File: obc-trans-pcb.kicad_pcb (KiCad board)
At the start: 4 copper layers, 95.9 x 90.2 mm, 31 parts, among them IC1 DS3234, J1 H1, J2 H2, J3 H_EPS, J4 DEBUGGING PORT, J5 PROGRAMMING PORT, SW1 SW_RST, U1 SN65HVD230, U2 ATMEGA32M1-MU, U3 SST25VF016B, U4 SST25VF016B, U5 SST25VF016B, Y1 8 MHz

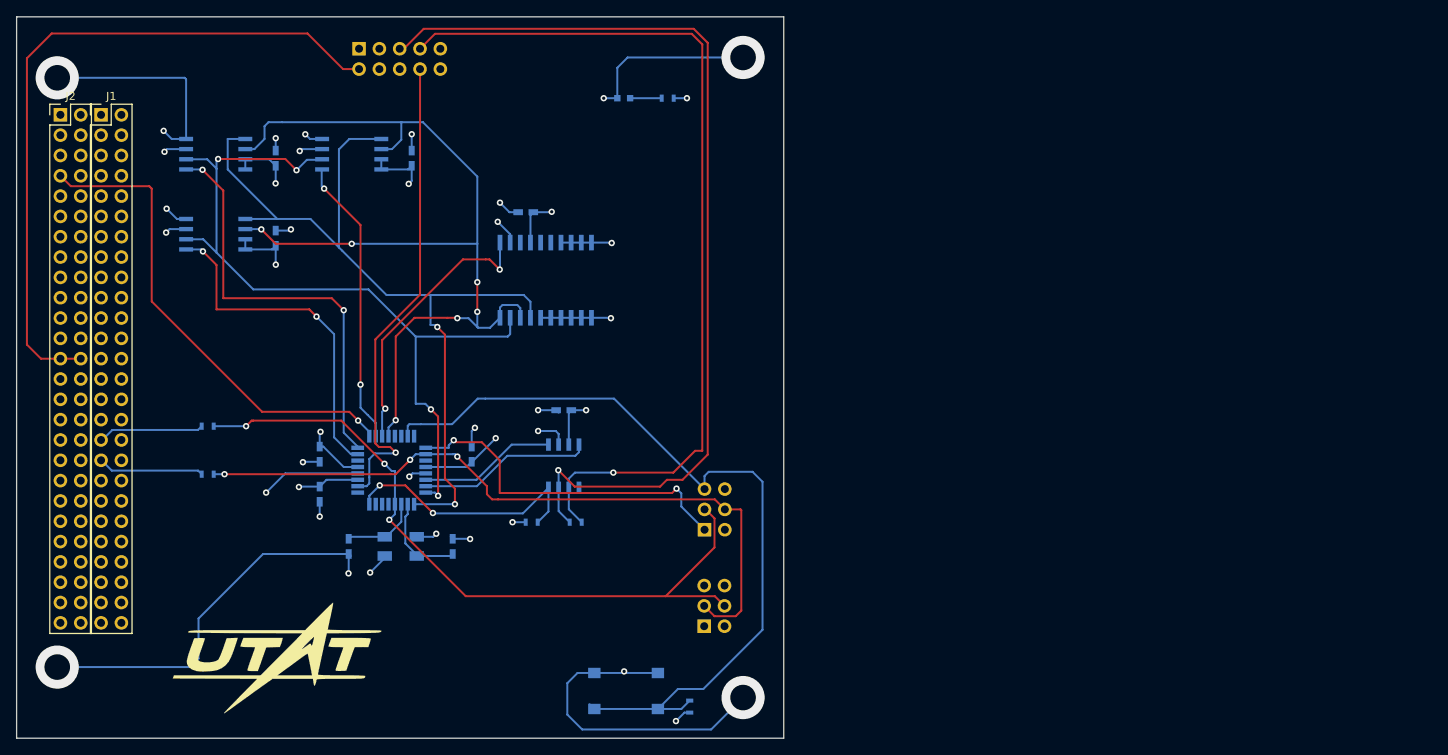
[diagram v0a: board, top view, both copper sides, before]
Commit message: Revert "vias smaller"
This reverts commit cac4902e6433adb27f0d020128540fc5646aa025.
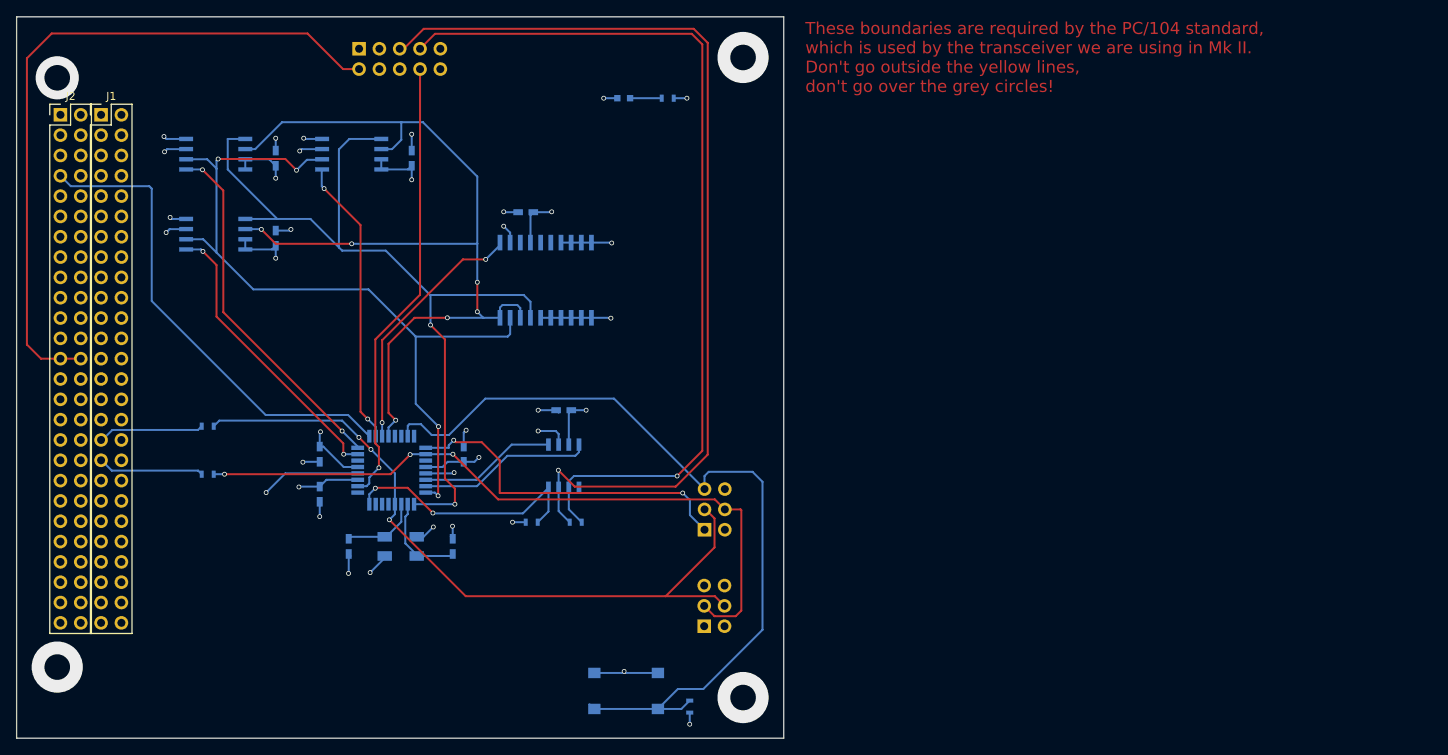
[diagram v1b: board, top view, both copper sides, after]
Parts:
- removed G***: LOGO, obc-trans-pcb:utat-logo
- moved C2 1.00 mm to (156.0, 104.5)
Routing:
- net GND: track 207.0 -> 83.2 mm
- net /CS_MEM2: track 52.8 -> 44.9 mm
- net /CS_MEM3: track 42.9 -> 36.6 mm
- net +3V3: track 73.4 -> 67.4 mm
- net /EPS_RST: track 60.4 -> 56.4 mm
- net /CS_RTC: track 35.4 -> 32.0 mm
- net /SCK: track 121.1 -> 119.0 mm
- net /RST: track 103.0 -> 104.1 mm
- net /MOSI_A: track 88.9 -> 87.9 mm
- net /MISO: track 101.4 -> 100.7 mm
- net /EN_UHF: track 60.7 -> 60.3 mm, vias 1 -> 0
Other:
- rule pad_to_mask_clearance: 0.25 -> 0.2
- board text added: "These boundaries are required by the PC/104 standard, which is used by the transceiver we are using in Mk II. Don't go outside the yellow lines, don't go over the grey circles!"

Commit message: vias smaller
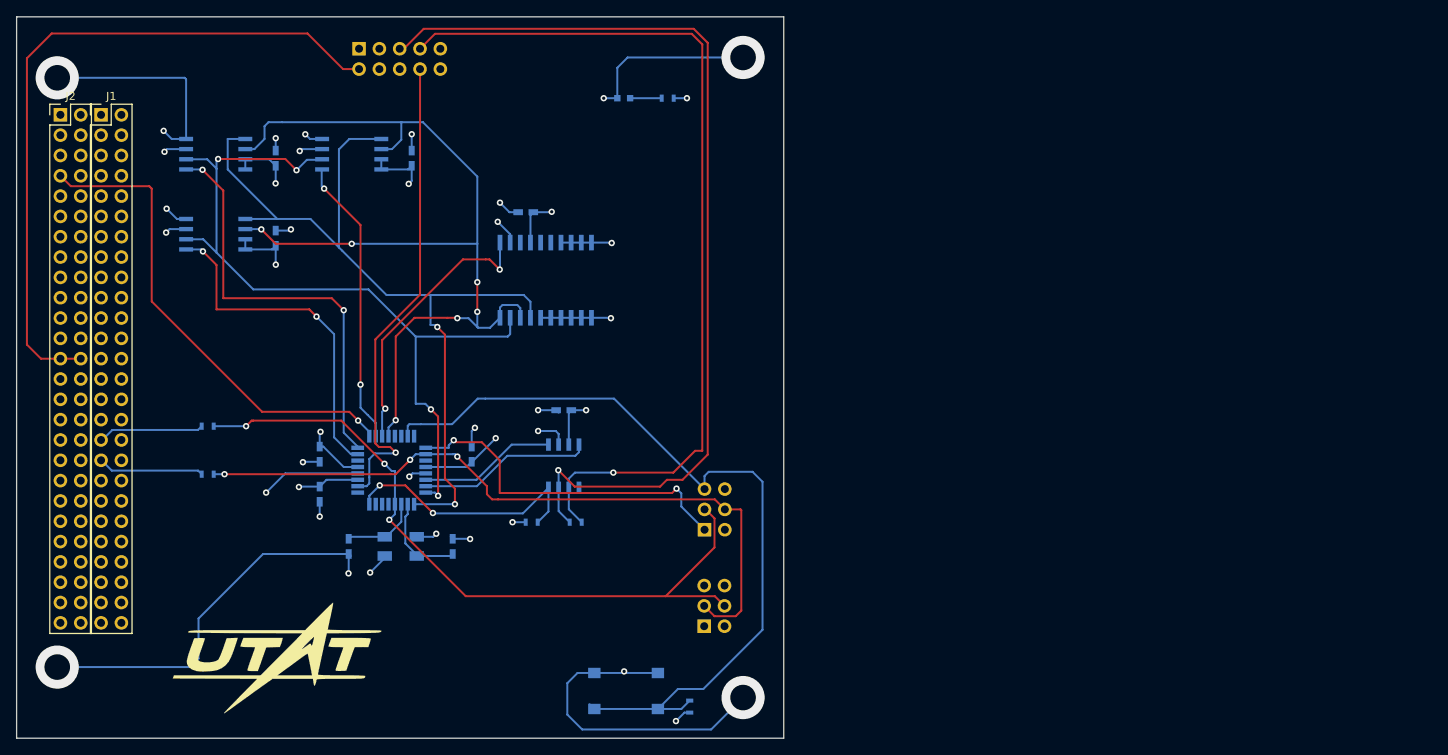
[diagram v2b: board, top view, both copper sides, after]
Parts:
- added G***: LOGO, obc-trans-pcb:utat-logo, F.Cu at (132.8, 129.6)
- moved C2 1.00 mm to (157.0, 104.5)
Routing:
- net GND: track 83.2 -> 207.0 mm
- net /CS_MEM2: track 44.9 -> 52.8 mm
- net /CS_MEM3: track 36.6 -> 42.9 mm
- net +3V3: track 67.4 -> 73.4 mm
- net /EPS_RST: track 56.4 -> 60.4 mm
- net /CS_RTC: track 32.0 -> 35.4 mm
- net /SCK: track 119.0 -> 121.1 mm
- net /RST: track 104.1 -> 103.0 mm
- net /MOSI_A: track 87.9 -> 88.9 mm
- net /MISO: track 100.7 -> 101.4 mm
- net /EN_UHF: track 60.3 -> 60.7 mm, vias 0 -> 1
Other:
- rule pad_to_mask_clearance: 0.2 -> 0.25
- board text removed: "These boundaries are required by the PC/104 standard, which is used by the transceiver we are using in Mk II. Don't go outside the yellow lines, don't go over the grey circles!"

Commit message: removed needless traces
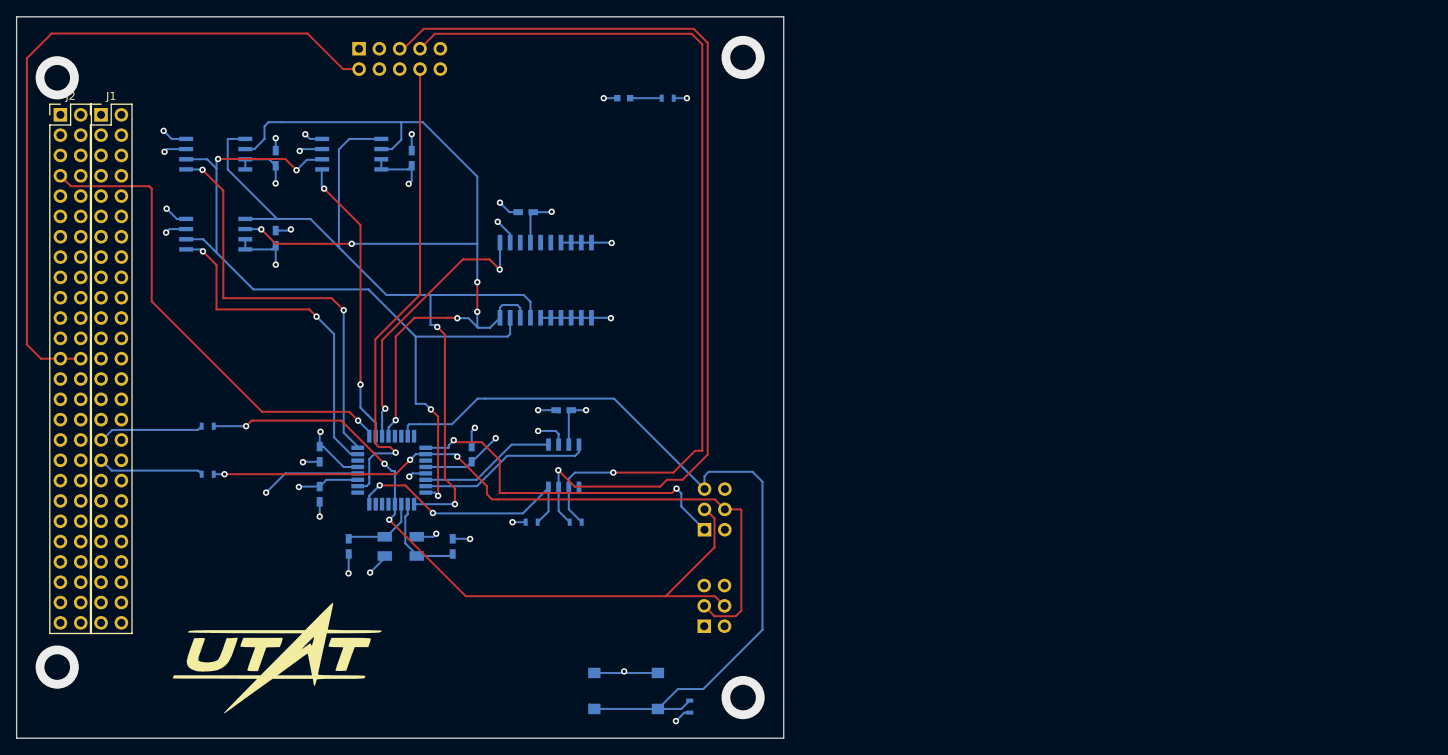
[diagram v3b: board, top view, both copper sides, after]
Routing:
- net GND: track 207.0 -> 87.3 mm
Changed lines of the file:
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@@
     (thickness 1.6)
     (drawings 4)
-    (tracks 494)
+    (tracks 478)
     (zones 0)
     (modules 31)
@@
   (gr_line (start 196 49.83) (end 100.11 49.83) (angle 90) (layer Edge.Cuts) (width 0.15))
   (gr_line (start 196 49.83) (end 196 140) (angle 90) (layer Edge.Cuts) (width 0.15))
-  (segment (start 141.625 116.975) (end 130.915 116.975) (width 0.25) (layer B.Cu) (net 1))
   (via (at 105.19 131.11) (size 5.4) (drill 3.2) (layers F.Cu B.Cu) (net 1))
-  (segment (start 121.78 131.11) (end 105.19 131.11) (width 0.25) (layer B.Cu) (net 1))
   (segment (start 122.85 130.04) (end 121.78 131.11) (width 0.25) (layer B.Cu) (net 1))
-  (segment (start 122.85 125.04) (end 122.85 130.04) (width 0.25) (layer B.Cu) (net 1))
-  (segment (start 130.915 116.975) (end 122.85 125.04) (width 0.25) (layer B.Cu) (net 1))
-  (segment (start 172.325 131.845554) (end 170.224446 131.845554) (width 0.25) (layer B.Cu) (net 1))
   (via (at 190.92 134.92) (size 5.4) (drill 3.2) (layers F.Cu B.Cu) (net 1))
-  (segment (start 186.93 138.91) (end 190.92 134.92) (width 0.25) (layer B.Cu) (net 1))
-  (segment (start 170.81 138.91) (end 186.93 138.91) (width 0.25) (layer B.Cu) (net 1))
-  (segment (start 168.95 137.05) (end 170.81 138.91) (width 0.25) (layer B.Cu) (net 1))
-  (segment (start 168.95 133.12) (end 168.95 137.05) (width 0.25) (layer B.Cu) (net 1))
-  (segment (start 170.224446 131.845554) (end 168.95 133.12) (width 0.25) (layer B.Cu) (net 1))
-  (segment (start 175.2 60) (end 175.2 56.2) (width 0.25) (layer B.Cu) (net 1))
   (via (at 190.92 54.91) (size 5.4) (drill 3.2) (layers F.Cu B.Cu) (net 1))
-  (segment (start 176.49 54.91) (end 190.92 54.91) (width 0.25) (layer B.Cu) (net 1))
-  (segment (start 175.2 56.2) (end 176.49 54.91) (width 0.25) (layer B.Cu) (net 1))
-  (segment (start 121.3 65.095) (end 121.3 57.64) (width 0.25) (layer B.Cu) (net 1))
   (via (at 105.19 57.45) (size 5.4) (drill 3.2) (layers F.Cu B.Cu) (net 1))
-  (segment (start 121.11 57.45) (end 105.19 57.45) (width 0.25) (layer B.Cu) (net 1))
-  (segment (start 121.3 57.64) (end 121.11 57.45) (width 0.25) (layer B.Cu) (net 1))
   (segment (start 161.805 78.05) (end 161.805 77.005) (width 0.25) (layer B.Cu) (net 1))
   (via (at 160.25 75.45) (size 0.8) (drill 0.4) (layers F.Cu B.Cu) (net 1))

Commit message: Revert "removed needless traces"
This reverts commit 13567706eda5130220792ebe949a07ef88a05d37.
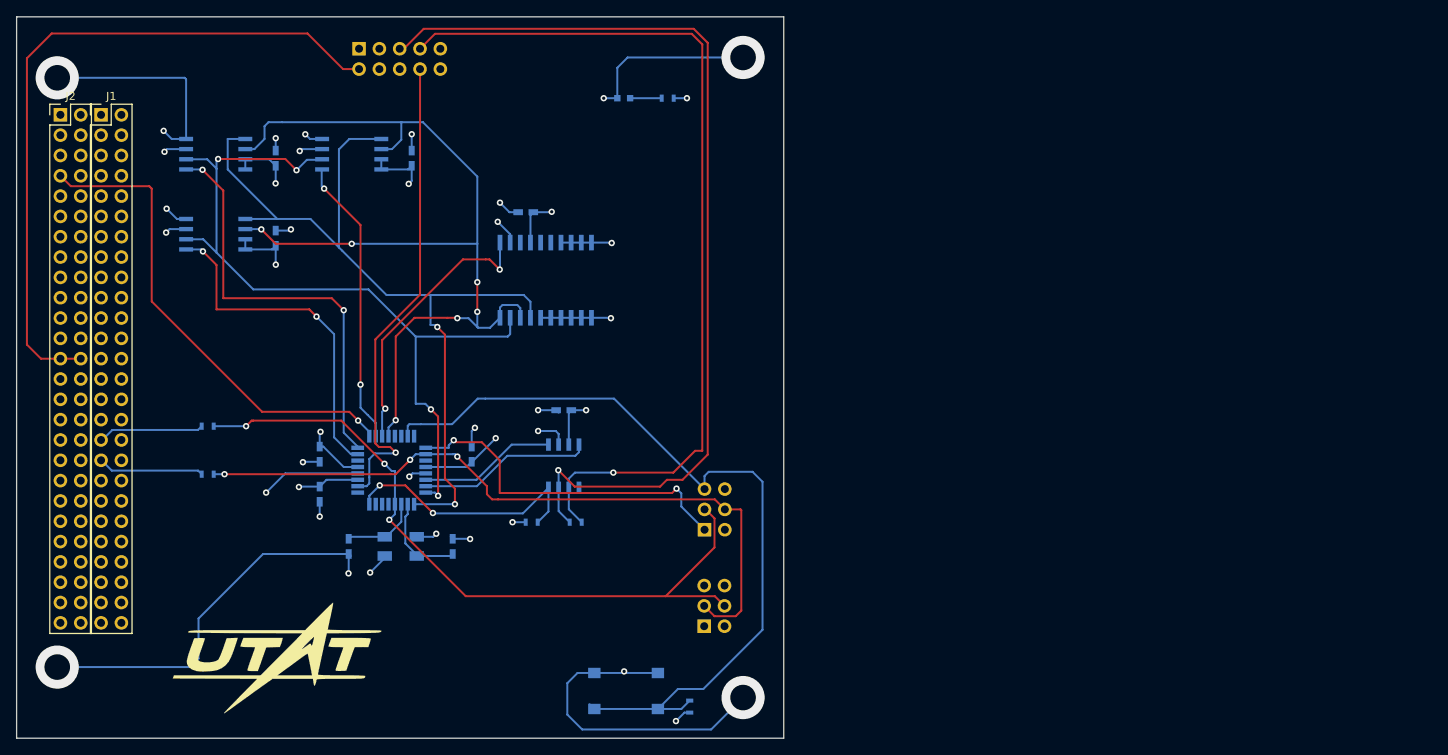
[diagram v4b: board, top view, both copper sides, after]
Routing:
- net GND: track 87.3 -> 207.0 mm
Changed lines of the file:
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@@
     (thickness 1.6)
     (drawings 4)
-    (tracks 478)
+    (tracks 494)
     (zones 0)
     (modules 31)
@@
   (gr_line (start 196 49.83) (end 100.11 49.83) (angle 90) (layer Edge.Cuts) (width 0.15))
   (gr_line (start 196 49.83) (end 196 140) (angle 90) (layer Edge.Cuts) (width 0.15))
+  (segment (start 141.625 116.975) (end 130.915 116.975) (width 0.25) (layer B.Cu) (net 1))
   (via (at 105.19 131.11) (size 5.4) (drill 3.2) (layers F.Cu B.Cu) (net 1))
+  (segment (start 121.78 131.11) (end 105.19 131.11) (width 0.25) (layer B.Cu) (net 1))
   (segment (start 122.85 130.04) (end 121.78 131.11) (width 0.25) (layer B.Cu) (net 1))
+  (segment (start 122.85 125.04) (end 122.85 130.04) (width 0.25) (layer B.Cu) (net 1))
+  (segment (start 130.915 116.975) (end 122.85 125.04) (width 0.25) (layer B.Cu) (net 1))
+  (segment (start 172.325 131.845554) (end 170.224446 131.845554) (width 0.25) (layer B.Cu) (net 1))
   (via (at 190.92 134.92) (size 5.4) (drill 3.2) (layers F.Cu B.Cu) (net 1))
+  (segment (start 186.93 138.91) (end 190.92 134.92) (width 0.25) (layer B.Cu) (net 1))
+  (segment (start 170.81 138.91) (end 186.93 138.91) (width 0.25) (layer B.Cu) (net 1))
+  (segment (start 168.95 137.05) (end 170.81 138.91) (width 0.25) (layer B.Cu) (net 1))
+  (segment (start 168.95 133.12) (end 168.95 137.05) (width 0.25) (layer B.Cu) (net 1))
+  (segment (start 170.224446 131.845554) (end 168.95 133.12) (width 0.25) (layer B.Cu) (net 1))
+  (segment (start 175.2 60) (end 175.2 56.2) (width 0.25) (layer B.Cu) (net 1))
   (via (at 190.92 54.91) (size 5.4) (drill 3.2) (layers F.Cu B.Cu) (net 1))
+  (segment (start 176.49 54.91) (end 190.92 54.91) (width 0.25) (layer B.Cu) (net 1))
+  (segment (start 175.2 56.2) (end 176.49 54.91) (width 0.25) (layer B.Cu) (net 1))
+  (segment (start 121.3 65.095) (end 121.3 57.64) (width 0.25) (layer B.Cu) (net 1))
   (via (at 105.19 57.45) (size 5.4) (drill 3.2) (layers F.Cu B.Cu) (net 1))
+  (segment (start 121.11 57.45) (end 105.19 57.45) (width 0.25) (layer B.Cu) (net 1))
+  (segment (start 121.3 57.64) (end 121.11 57.45) (width 0.25) (layer B.Cu) (net 1))
   (segment (start 161.805 78.05) (end 161.805 77.005) (width 0.25) (layer B.Cu) (net 1))
   (via (at 160.25 75.45) (size 0.8) (drill 0.4) (layers F.Cu B.Cu) (net 1))
